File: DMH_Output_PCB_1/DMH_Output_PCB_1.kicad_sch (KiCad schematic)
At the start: 0 parts

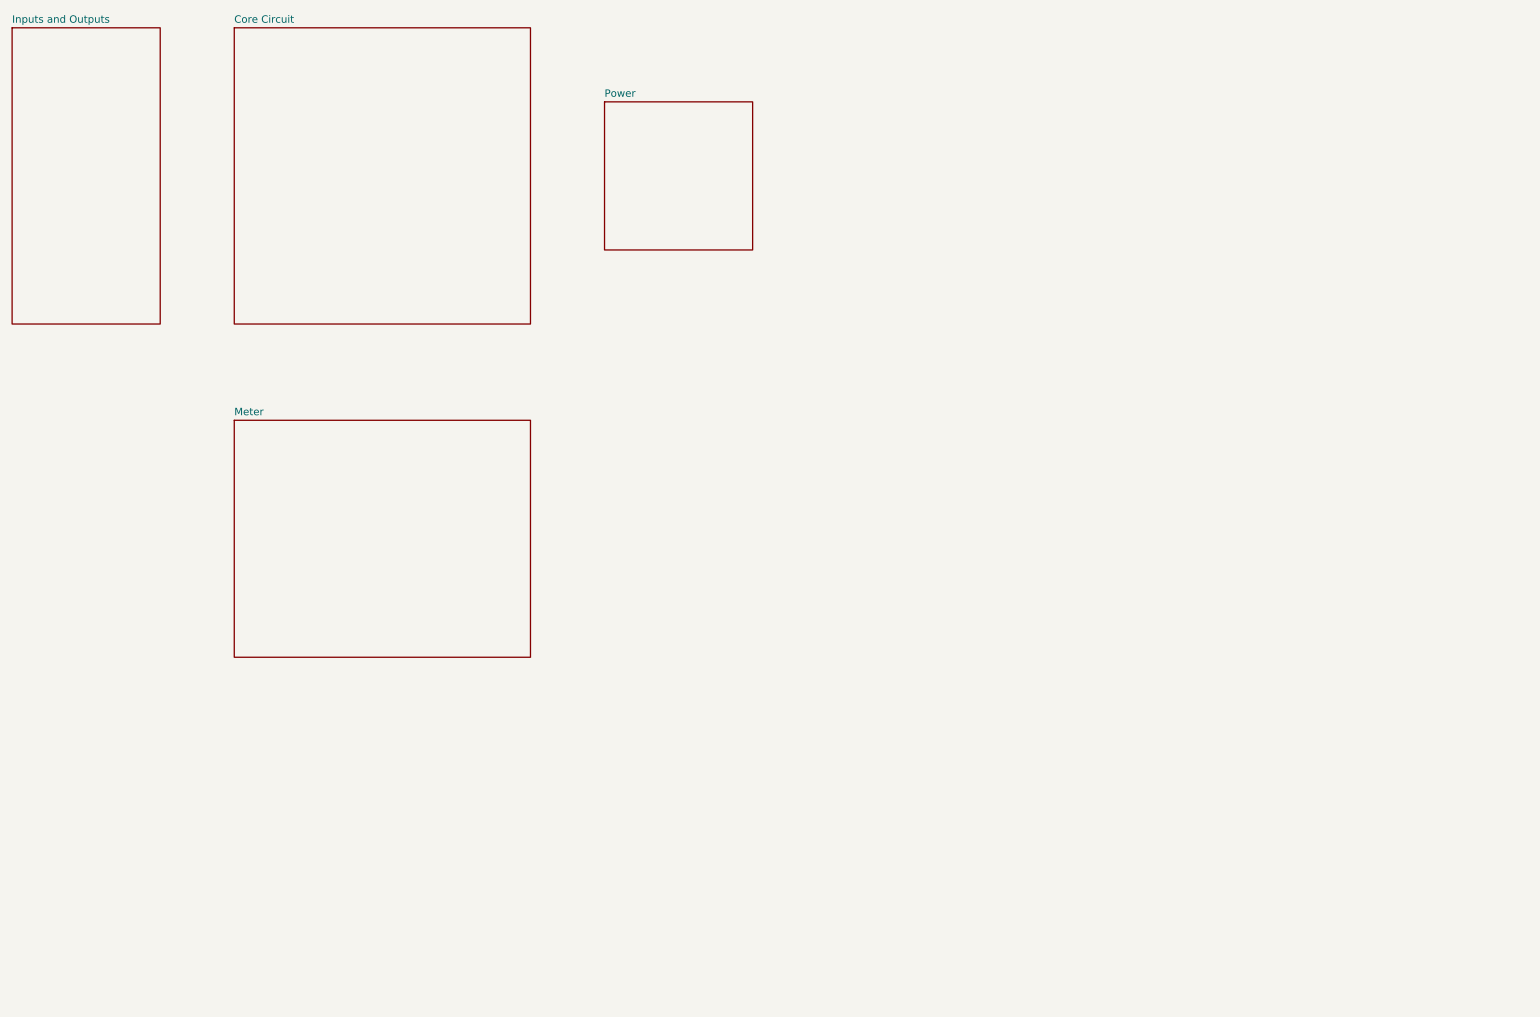
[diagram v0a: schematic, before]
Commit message: Schematic in progress
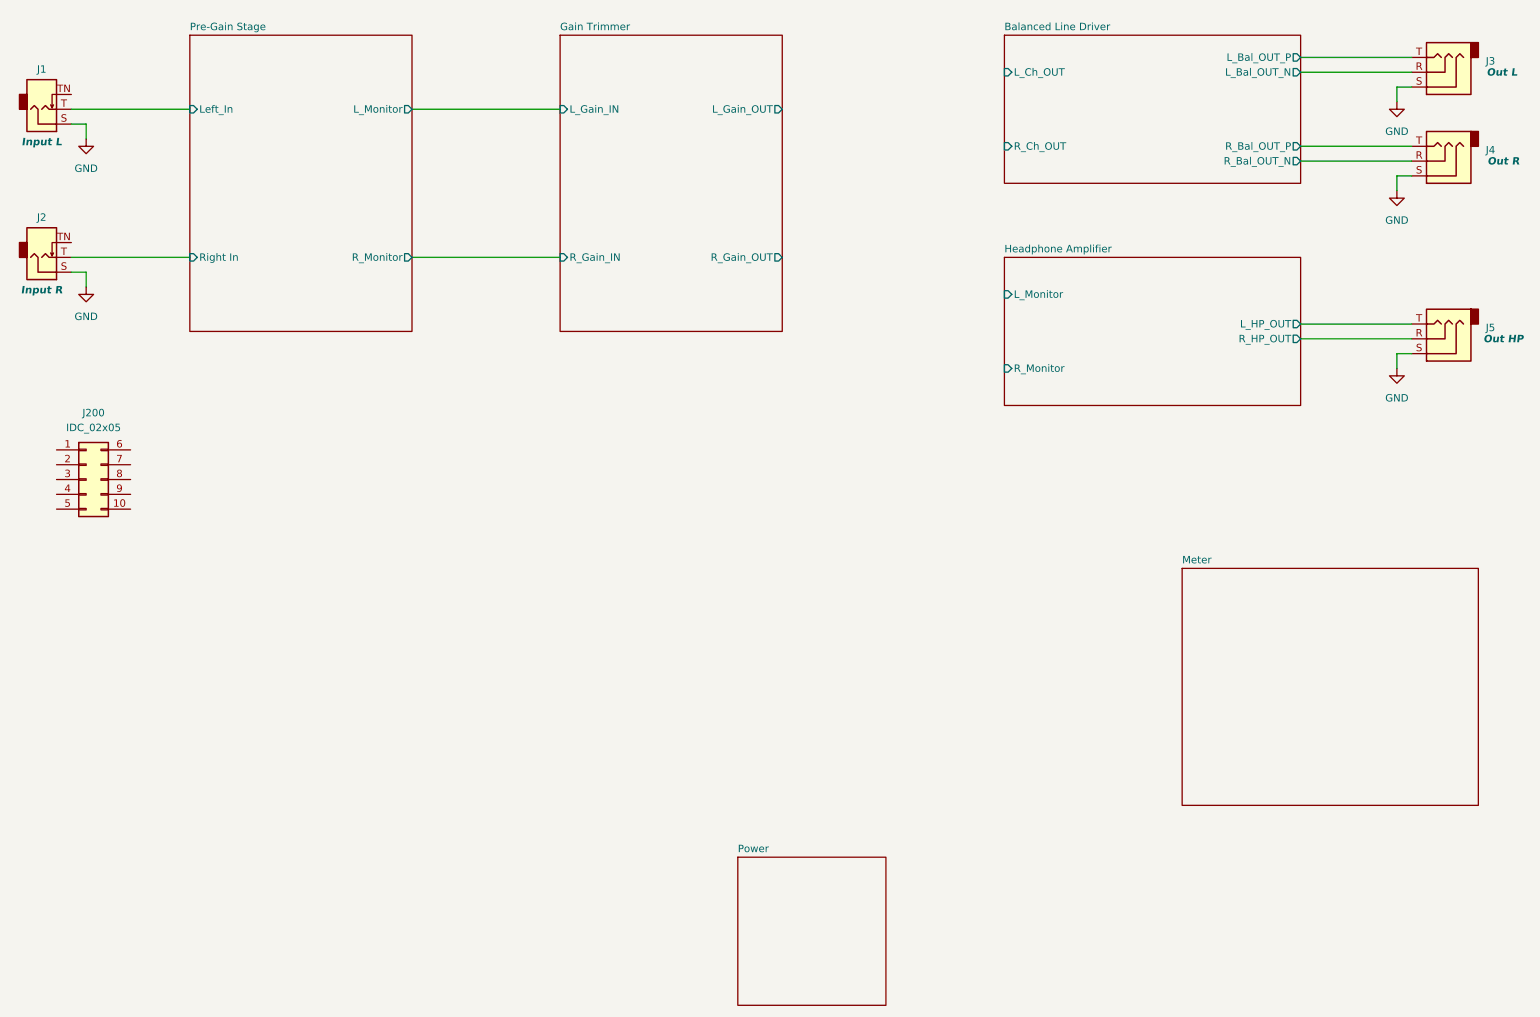
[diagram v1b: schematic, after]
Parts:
- added J1, J2: TS_Jack_6.35mm_Sw, SynthStuff:CUI_MJ-63052A, symbol SynthStuff:TS_Jack_6.35mm_Sw
- added J200: IDC_02x05, SynthStuff:IDC-Header_2x05_P2.54mm_Vertical_BackBone, symbol SynthStuff:BackBone_Connector_10Pin
- added J3, J4, J5: AudioJack3, symbol Connector_Audio:AudioJack3
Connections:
- new net Balanced Line Driver/L_Bal_OUT_N: J3.R
- new net Balanced Line Driver/L_Bal_OUT_P: J3.T
- new net Balanced Line Driver/R_Bal_OUT_N: J4.R
- new net Balanced Line Driver/R_Bal_OUT_P: J4.T
- new net GND: J1.S, J2.S, J3.S, J4.S, J5.S
- new net Headphone Amplifier/L_HP_OUT: J5.T
- new net Headphone Amplifier/R_HP_OUT: J5.R
- new net Pre-Gain Stage/Left_In: J1.T
- new net Pre-Gain Stage/Right In: J2.T
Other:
- removed sheet Core Circuit
- removed sheet Inputs and Outputs
- added sheet Balanced Line Driver (Balanced_line_driver.kicad_sch)
- added sheet Gain Trimmer (Gain_trimmer.kicad_sch)
- added sheet Headphone Amplifier (Headphone_amplifier.kicad_sch)
- added sheet Pre-Gain Stage (Pregain_stage.kicad_sch)
